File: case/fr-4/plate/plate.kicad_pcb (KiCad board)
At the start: 2 copper layers, 152.4 x 104.6 mm, 34 parts

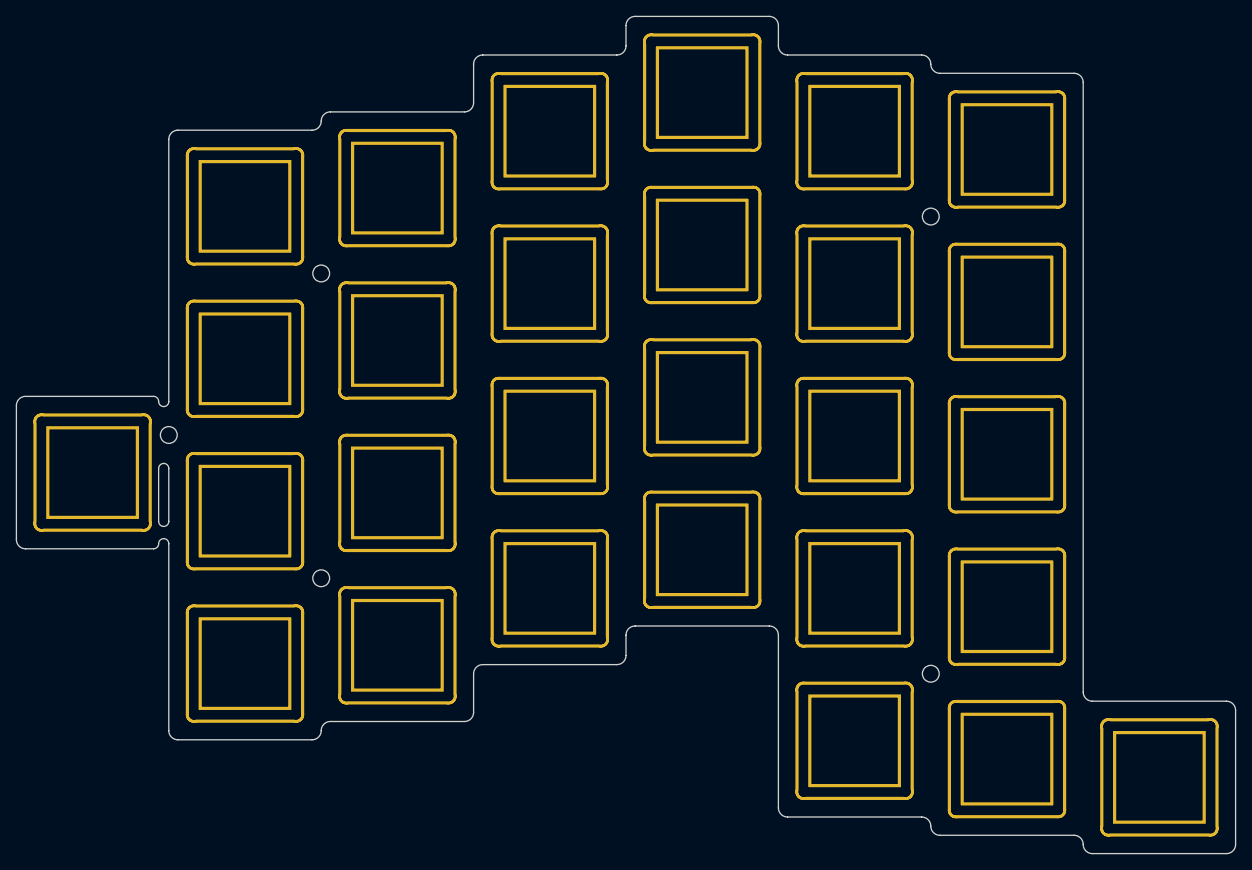
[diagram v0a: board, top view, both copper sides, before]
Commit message: Fill all zones
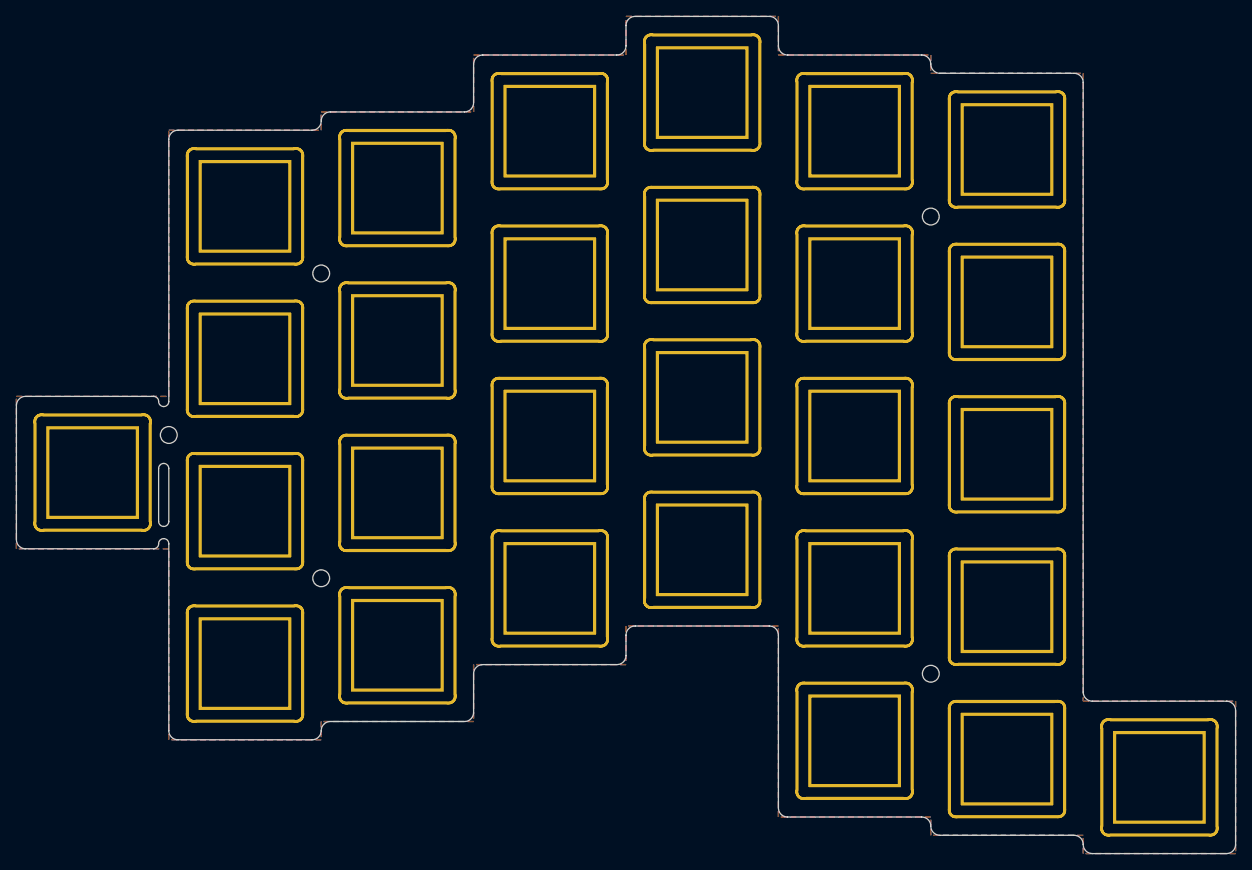
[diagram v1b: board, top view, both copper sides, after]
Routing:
- added copper zone on B.Cu, net (none)
- added copper zone on F.Cu, net (none)
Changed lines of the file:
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@@
   (gr_arc (start 88.392 105.156) (end 87.757004 105.156) (angle 90) (layer "Edge.Cuts") (width 0.1))
   (gr_line (start 203.327 56.896) (end 203.327 133.096) (layer "Edge.Cuts") (width 0.1))
+  (zone (net 0) (net_name "") (layer "F.Cu") (hatch edge 0.508)
+    (connect_pads (clearance 0.508))
+    (min_thickness 0.254) (filled_areas_thickness no)
+    (fill yes (thermal_gap 0.508) (thermal_bridge_width 0.508))
+    (polygon
+      (pts
+        (xy 165.227 53.467)
+        (xy 184.277 53.467)
+        (xy 184.277 55.753)
+        (xy 203.327 55.753)
+        (xy 203.327 134.239)
+        (xy 222.377 134.239)
+        (xy 222.377 153.289)
+        (xy 203.327 153.289)
+        (xy 203.327 151.003)
+        (xy 184.277 151.003)
+        (xy 184.277 148.717)
+        (xy 165.227 148.717)
+        (xy 165.227 124.841)
+        (xy 146.177 124.841)
+        (xy 146.177 129.667)
+        (xy 127.127 129.667)
+        (xy 127.127 136.779)
+        (xy 108.077 136.779)
+        (xy 108.077 139.065)
+        (xy 89.027 139.065)
+        (xy 89.027 115.189)
+        (xy 69.977 115.189)
+        (xy 69.977 96.139)
+        (xy 89.027 96.139)
+        (xy 89.027 62.865)
+        (xy 108.077 62.865)
+        (xy 108.077 60.579)
+        (xy 127.127 60.579)
+        (xy 127.127 53.467)
+        (xy 146.177 53.467)
+        (xy 146.177 48.641)
+        (xy 165.227 48.641)
+      )
+    )
+  )
+  (zone (net 0) (net_name "") (layer "B.Cu") (hatch edge 0.508)
+    (connect_pads (clearance 0.508))
+    (min_thickness 0.254) (filled_areas_thickness no)
+    (fill yes (thermal_gap 0.508) (thermal_bridge_width 0.508))
+    (polygon
+      (pts
+        (xy 165.227 53.467)
+        (xy 184.277 53.467)
+        (xy 184.277 55.753)
+        (xy 203.327 55.753)
+        (xy 203.327 134.239)
+        (xy 222.377 134.239)
+        (xy 222.377 153.289)
+        (xy 203.327 153.289)
+        (xy 203.327 151.003)
+        (xy 184.277 151.003)
+        (xy 184.277 148.717)
+        (xy 165.227 148.717)
+        (xy 165.227 124.841)
+        (xy 146.177 124.841)
+        (xy 146.177 129.667)
+        (xy 127.127 129.667)
+        (xy 127.127 136.779)
+        (xy 108.077 136.779)
+        (xy 108.077 139.065)
+        (xy 89.027 139.065)
+        (xy 89.027 115.189)
+        (xy 69.977 115.189)
+        (xy 69.977 96.139)
+        (xy 89.027 96.139)
+        (xy 89.027 62.865)
+        (xy 108.077 62.865)
+        (xy 108.077 60.579)
+        (xy 127.127 60.579)
+        (xy 127.127 53.467)
+        (xy 146.177 53.467)
+        (xy 146.177 48.641)
+        (xy 165.227 48.641)
+      )
+    )
+  )
 )
